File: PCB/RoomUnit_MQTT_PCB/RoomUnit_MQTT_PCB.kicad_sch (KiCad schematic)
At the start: 26 parts, among them J1 Conn_01x08_Socket, Q1 MMBTA06, U1 LMV393, U2 MOUDLE-SEEEDUINO-XIAO-ESP32C3, U3 L78L24_SOT89

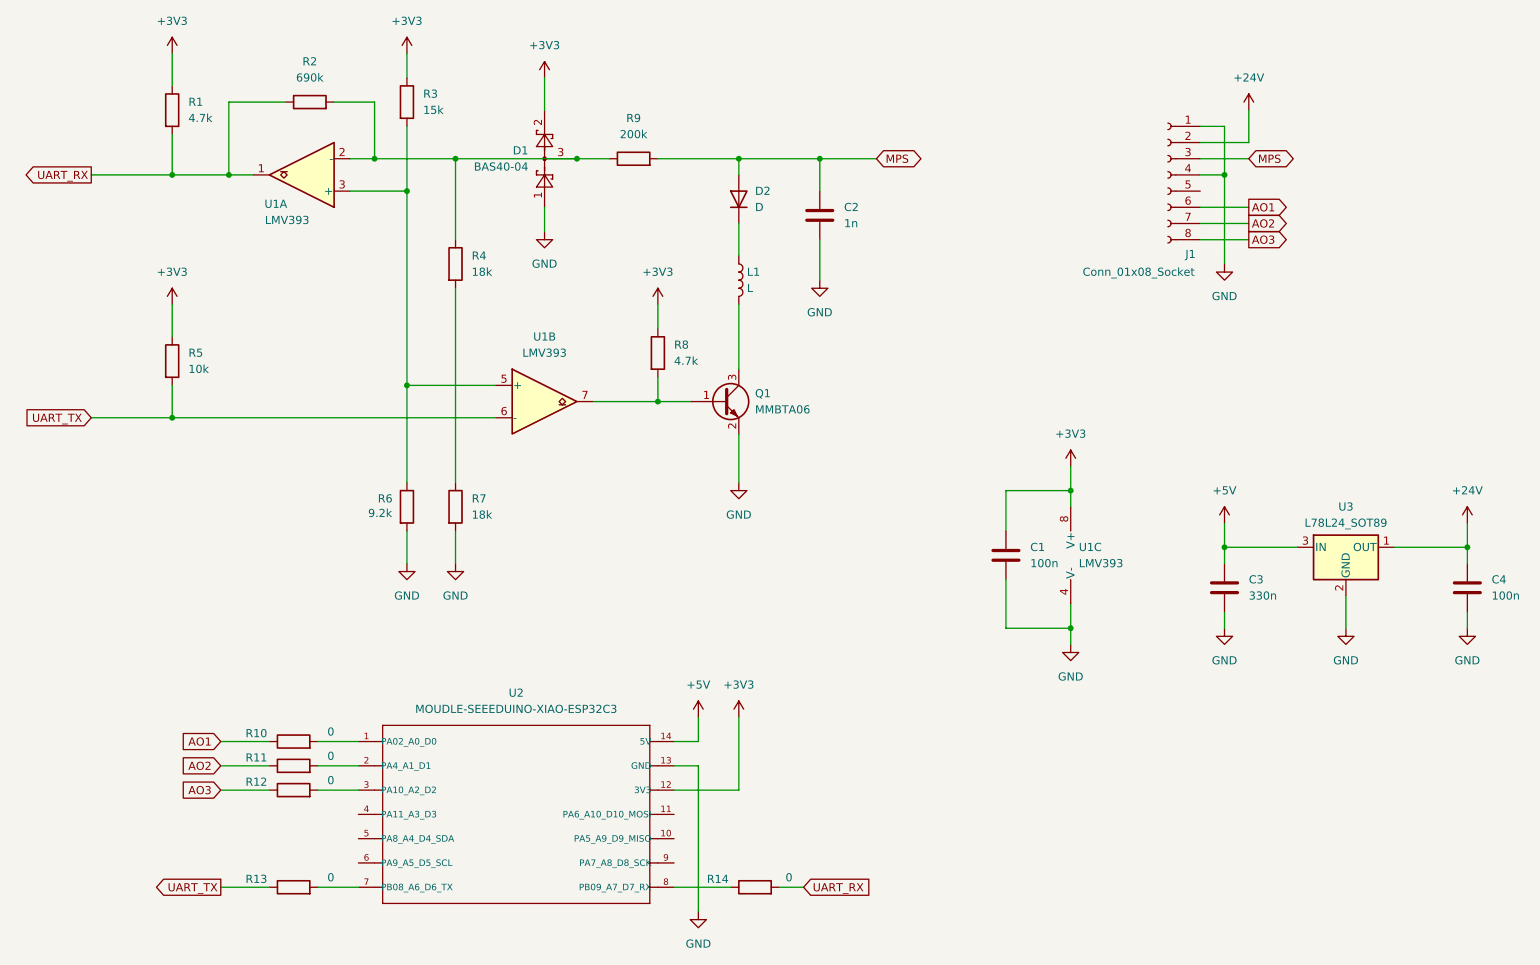
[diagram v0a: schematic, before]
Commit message: pcb progress
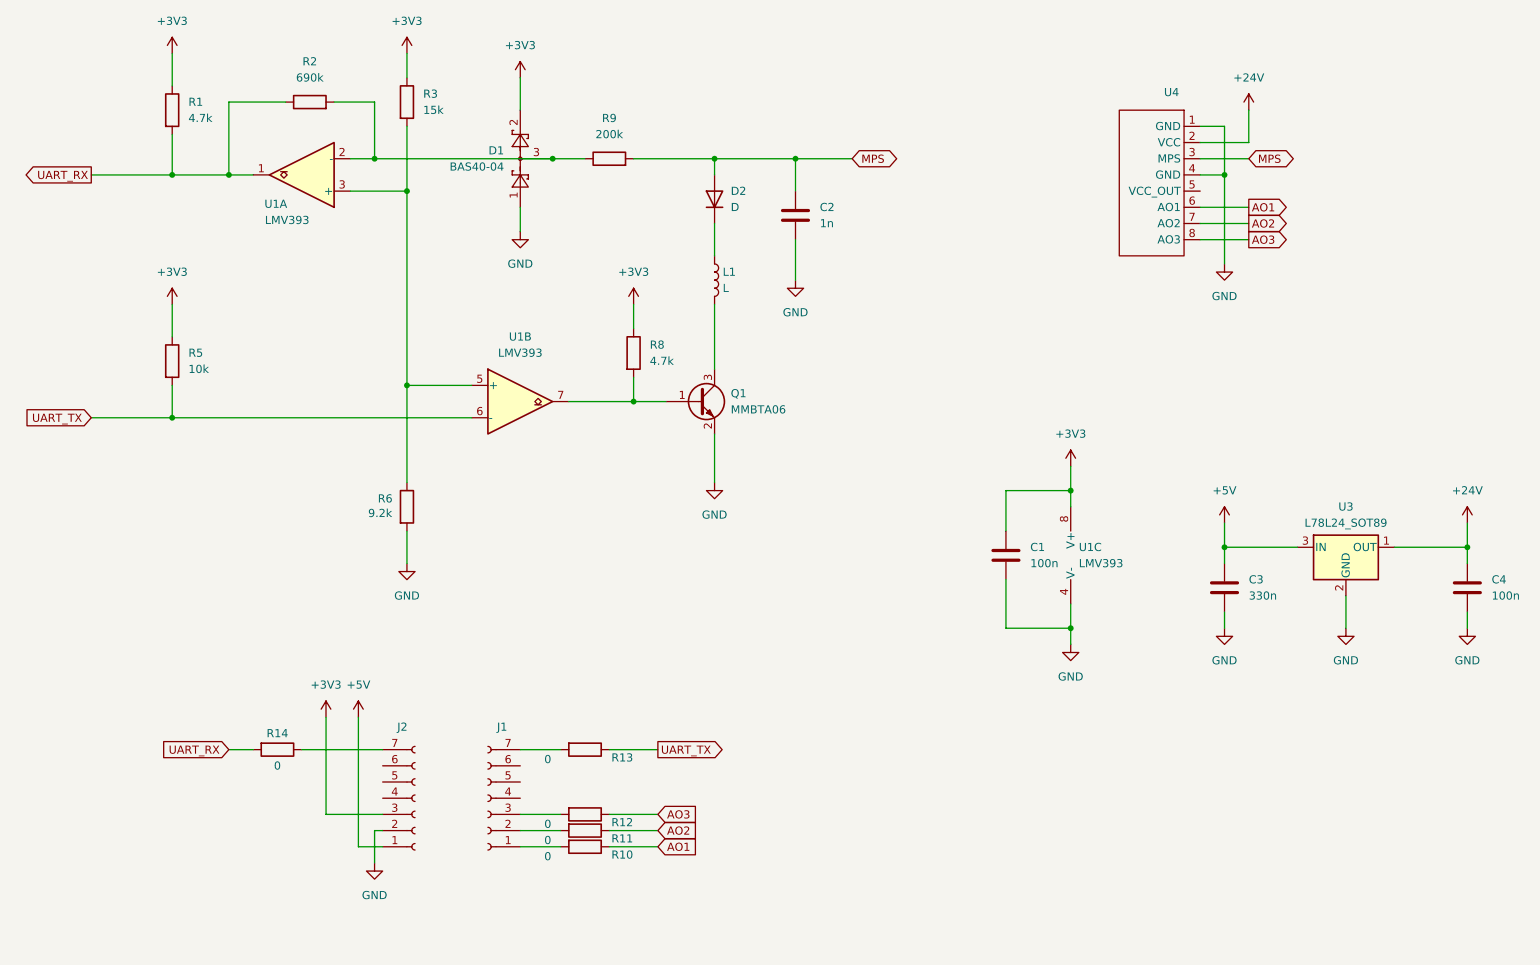
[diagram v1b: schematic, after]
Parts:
- removed J1: Conn_01x08_Socket, Connector_Samtec_HPM_THT:Samtec_HPM-08-01-x-S_Straight_1x08_Pitch5.08mm, symbol Connector:Conn_01x08_Socket
- removed R4, R7: 18k, Resistor_SMD:R_0805_2012Metric_Pad1.20x1.40mm_HandSolder, symbol Device:R
- removed U2: MOUDLE-SEEEDUINO-XIAO-ESP32C3, RF_Module:MCU_Seeed_ESP32C3, symbol Seeed studio:MOUDLE-SEEEDUINO-XIAO-ESP32C3
- added J1, J2: Conn_01x07_Socket, Project_Library:XIAO_ESP32-C3_Custom_Connector, symbol Connector:Conn_01x07_Socket
- added U4: ~, Project_Library:RoomUnit_Connector_5mm, symbol Project_Library:RoomUnit_Connector
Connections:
- net +24V: now also U4.2 (VCC)
- net +3V3: now also J2.3 (Pin_3)
- net +5V: now also J2.1 (Pin_1)
- net AO1: now also U4.6 (AO1)
- net AO2: now also U4.7 (AO2)
- net AO3: now also U4.8 (AO3)
- net GND: now also J2.2 (Pin_2), U4.1 (GND), U4.4 (GND)
- net MPS: now also U4.3 (MPS)
- net at R10.2: now also J1.1 (Pin_1)
- net at R12.2: now also J1.3 (Pin_3)
- net at R11.2: now also J1.2 (Pin_2)
- net at R13.2: now also J1.7 (Pin_7)
- net at R14.1: now also J2.7 (Pin_7)
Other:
- moved on the sheet: C2, D1, D2, L1, Q1, R10, R11, R12, R13, R14, R8, R9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
